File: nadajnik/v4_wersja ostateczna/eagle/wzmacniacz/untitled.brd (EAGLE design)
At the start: 86.3 x 42.9 mm, 26 parts, among them IC1 LM358N, M1 ELECTRET_MICROPHON-F6050AP, T1 BF199

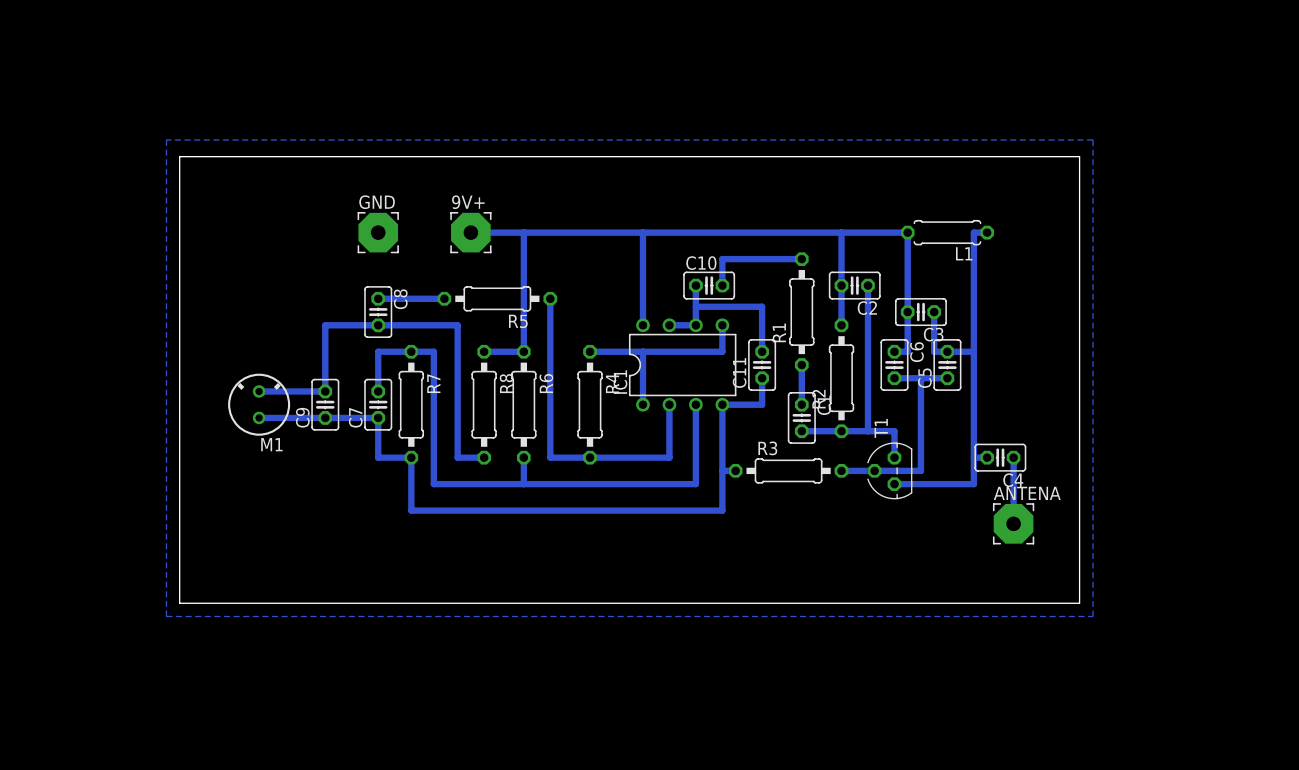
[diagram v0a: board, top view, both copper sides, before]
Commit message: poprawa nadajnika
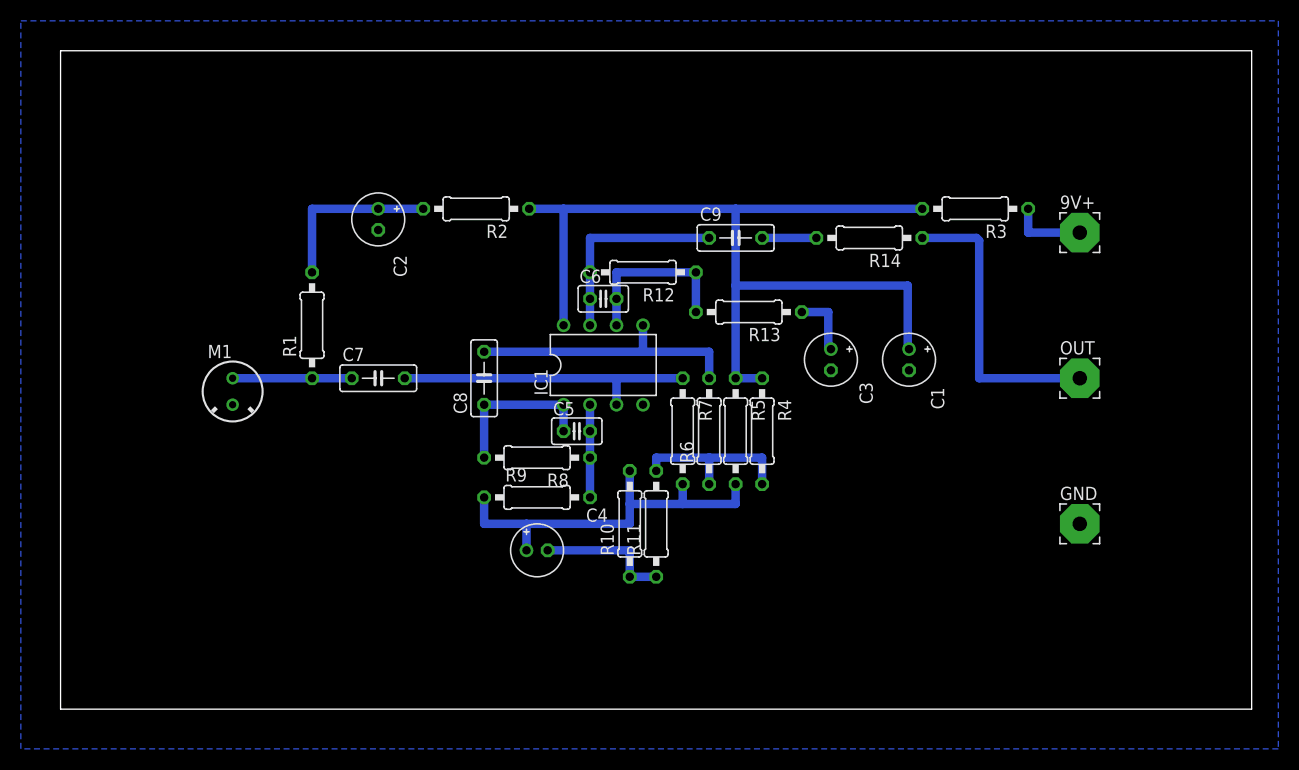
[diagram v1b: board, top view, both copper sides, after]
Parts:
- removed ANTENA: (no value), wirepad:3,81/1,4
- removed C10: 22u, rcl:C025-025X050
- removed C11: 1n, rcl:C025-025X050
- removed L1: (no value), rcl:0207/7
- removed T1: BF199, transistor-npn:TO92
- added OUT: (no value), wirepad:3,81/1,4
- added R10, R11, R14: 10k, rcl:0207/10
- added R12: 39k, rcl:0207/10
- added R13, R9: 5.7k, rcl:0207/10
- C1: value 47n -> 100u; device rcl:C025-025X050 -> rcl:E2-5
- C2: value 1n -> 100u; device rcl:C025-025X050 -> rcl:E2-5
- C3: value 39p -> 100u; device rcl:C025-025X050 -> rcl:E2-5
- C4: value 2p -> 100u; device rcl:C025-025X050 -> rcl:E2-5
- C5: value 5p -> 470p
- C6: value 68p -> 470p
- C7, C9: value 1n -> 220n; device rcl:C025-025X050 -> rcl:C050-025X075
- C8: value 10u -> 220n; device rcl:C025-025X050 -> rcl:C050-025X075
- R1: value 220 -> 2.2k
- R2: value 33k -> 1k
- R3: value 150Ω -> 100
- R4: value 150k -> 10k
- R5: value 300 -> 10k
- R6: value 4.7k -> 10k
- R7: value 4.7 -> 10k
- R8: value 1.8k -> 47k
- moved GND 72.9 mm to (86.4, 7.62)
- moved 9V+ 58.4 mm to (86.4, 35.6)
- moved R1 47.0 mm to (12.7, 26.7)
- moved C2 46.2 mm to (19.1, 36.8), turned to 270 degrees
- moved C4 45.3 mm to (34.3, 5.08), turned to 0 degrees
- moved C9 42.5 mm to (53.3, 35.1), turned to 0 degrees
- moved R2 38.6 mm to (28.4, 37.8), turned to 180 degrees
- moved C5 36.1 mm to (38.1, 16.5), turned to 0 degrees
- moved R3 30.9 mm to (76.3, 37.8), turned to 180 degrees
- moved C6 28.7 mm to (40.6, 29.2), turned to 0 degrees
- moved R7 26.2 mm to (48.3, 16.5)
- moved R5 26.2 mm to (53.3, 16.5), turned to 270 degrees
- moved R6 18.0 mm to (50.8, 16.5), turned to 90 degrees
- moved R4 16.7 mm to (55.9, 16.5)
- moved C8 12.0 mm to (29.2, 21.6), turned to 90 degrees
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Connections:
- new net N$12: C3.+, R13.1
- new net N$15: C9.2, R14.2
- net GND: now also C1.-, C2.-, C3.-, C4.-, M1.2, R10.1, R11.1; no longer C11.1, C7.1, C9.1, M1.1, R3.1, R7.2
- net N$1: now also C7.2, IC1.3, R7.1; no longer C10.2, R1.2
- net N$10: now also 9V+.1, R3.1; no longer IC1.2, R4.2, R5.1
- net N$11: now also C6.2, IC1.6, R12.1, R13.2; no longer C7.2, IC1.3, R6.2, R7.1
- net N$13: now also C6.1, C9.1, IC1.7, R12.2; no longer C8.1, R5.2
- net N$14: now also OUT.1, R14.1; no longer C8.2, C9.2, M1.2, R8.2
- net N$2: now also C5.1, C8.1, IC1.1, R8.2; no longer C1.1, R1.1
- net N$3: now also C5.2, IC1.2, R8.1, R9.2; no longer C1.2, C2.1, R2.1, T1.1
- net N$4: now also C4.+, R10.2, R5.2, R7.2, R9.1; no longer C10.1, C11.2, IC1.6, IC1.7
- net N$5: now also C8.2, IC1.5, R6.2; no longer C5.1, C6.2, R3.2, T1.2
- net N$6: now also R11.2, R4.2, R6.1; no longer C3.1, C4.2, C5.2, L1.1, T1.3
- net N$7: now also C7.1, M1.1, R1.1; no longer 9V+.1, C2.2, C3.2, C6.1, IC1.8, L1.2, R2.2, R6.1, R8.1
- net N$8: now also C2.+, R1.2, R2.2; no longer ANTENA.1, C4.1
- net N$9: now also C1.+, IC1.8, R2.1, R3.2, R5.1; no longer IC1.1, IC1.5
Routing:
- net N$7: track 87.6 -> 11.4 mm
- net N$9: track 20.3 -> 90.5 mm
- net GND: track 71.1 -> 13.0 mm
- net N$11: track 57.1 -> 16.5 mm
- net N$6: track 41.9 -> 16.5 mm
- net N$10: track 31.8 -> 7.24 mm
- net N$4: track 17.0 -> 38.1 mm
- net N$1: track 10.2 -> 29.2 mm
- net N$3: track 25.4 -> 8.89 mm
- net N$13: track 6.35 -> 19.8 mm
- net N$14: track 40.6 -> 28.4 mm
- net N$2: track 3.81 -> 15.2 mm
- net N$8: track 6.35 -> 16.8 mm
- net N$12: track 0.00 -> 6.20 mm
- net N$15: track 0.00 -> 5.21 mm
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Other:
- board size 86.3 x 42.9 mm -> 114.3 x 63.2 mm
